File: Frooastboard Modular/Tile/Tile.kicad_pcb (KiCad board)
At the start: 4 copper layers, 91.1 x 79.6 mm, 192 parts, among them J1 Conn_01x08, J10 Conn_01x02, J2 Conn_01x06, J3 Conn_01x06, J4 Conn_01x10, J5 Conn_01x12, J6 SW Interface, J7 Conn_01x04, J8 Conn_01x08, J9 Conn_01x05, U1 IS31FL3733-QF, U2 RP2040, U3 W25Q32JVZP, U4 LM317L_SOT-89, Y1 12MHz

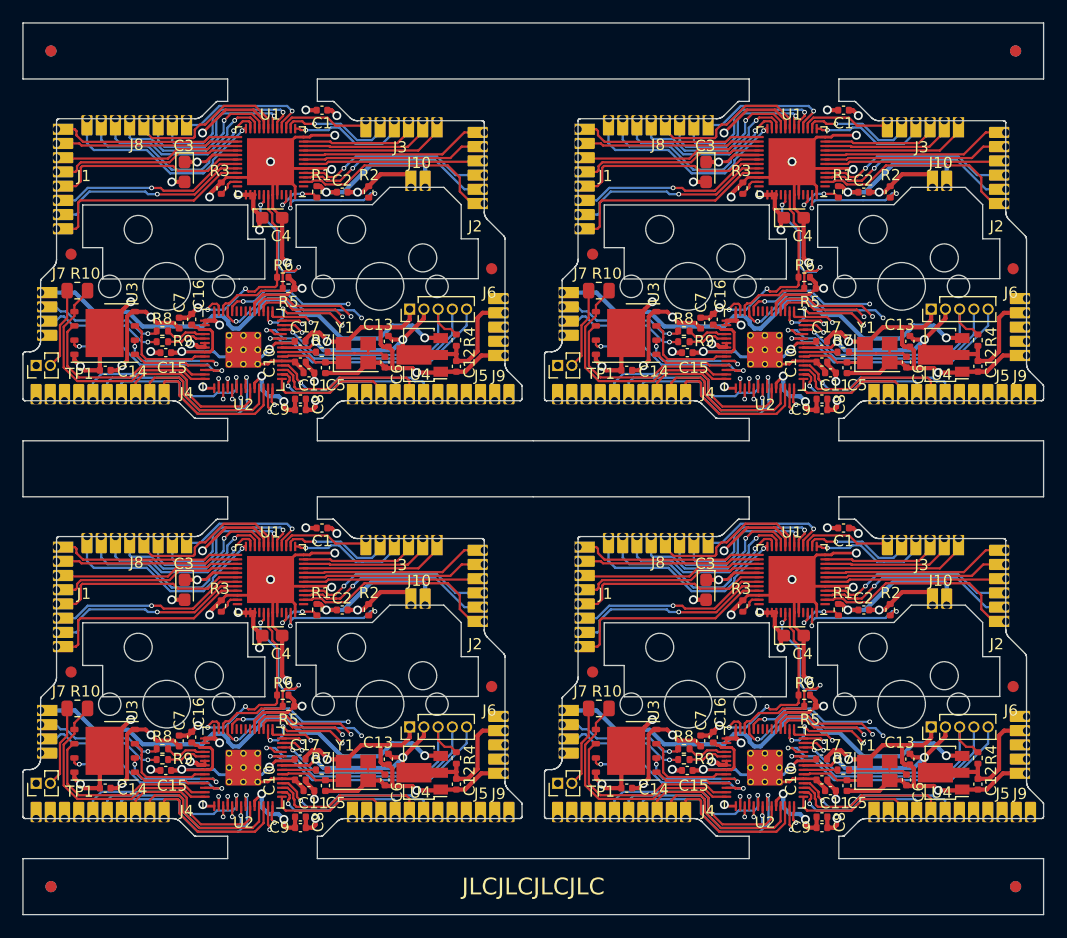
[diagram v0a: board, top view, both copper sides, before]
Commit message: stuff
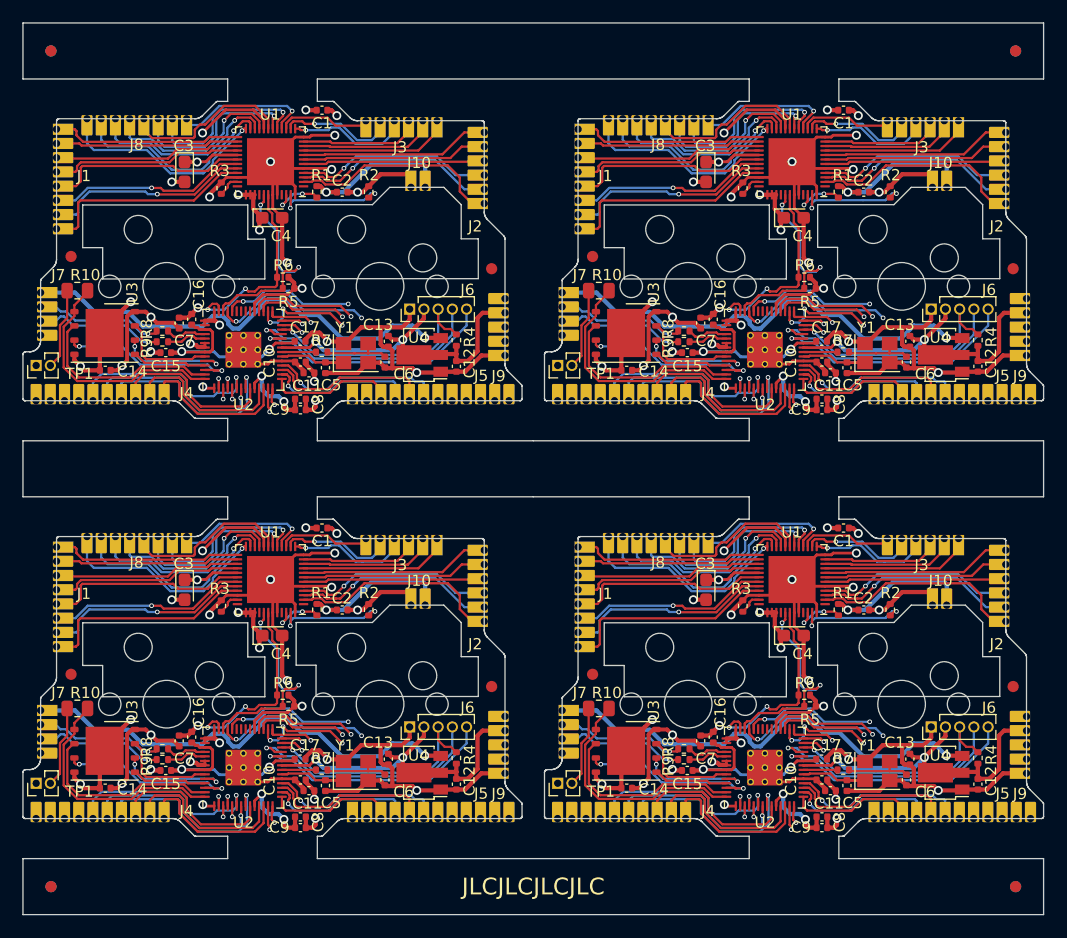
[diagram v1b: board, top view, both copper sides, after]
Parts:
- removed the REF** at (110.3, 77.9)
- removed the REF** at (148.1, 22.5) (x2)
- removed the REF** at (148.1, 97.1) (x2)
- removed the REF** at (61.9, 22.5) (x2)
- removed the REF** at (61.9, 97.1) (x2)
- removed the REF** at (110.3, 40.6)
- removed the REF** at (63.7, 77.9)
- removed the REF** at (63.7, 40.6)
- added REF**: Fiducial_1mm_Mask2mm, Fiducial:Fiducial_1mm_Mask2mm, F.Cu at (110.3, 78.1)
- added REF**: Fiducial_1mm_Mask2mm, Fiducial:Fiducial_1mm_Mask2mm, F.Cu at (63.7, 78.1)
- added REF**: Fiducial, Fiducial, F.Cu at (61.9, 97.1)
- added REF**: Fiducial, Fiducial, B.Cu at (61.9, 22.5)
- added REF**: Fiducial, Fiducial, B.Cu at (148.1, 22.5)
- added REF**: Fiducial, Fiducial, B.Cu at (148.1, 97.1)
- added REF**: Fiducial_1mm_Mask2mm, Fiducial:Fiducial_1mm_Mask2mm, F.Cu at (63.7, 40.8)
- added REF**: Fiducial, Fiducial, B.Cu at (61.9, 97.1)
- added REF**: Fiducial, Fiducial, F.Cu at (148.1, 22.5)
- added REF**: Fiducial, Fiducial, F.Cu at (148.1, 97.1)
- added REF**: Fiducial, Fiducial, F.Cu at (61.9, 22.5)
- added REF**: Fiducial_1mm_Mask2mm, Fiducial:Fiducial_1mm_Mask2mm, F.Cu at (110.3, 40.8)
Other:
- board text removed: "V-CUT"
